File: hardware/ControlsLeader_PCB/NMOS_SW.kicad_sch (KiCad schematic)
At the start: 7 parts, among them Q15 NMOS

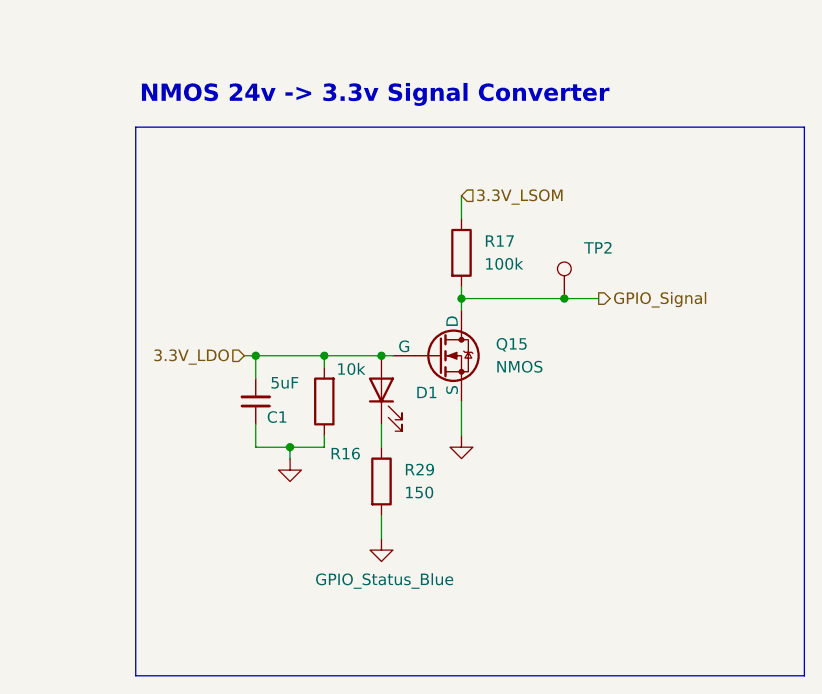
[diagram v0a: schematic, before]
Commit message: Schematic RevA
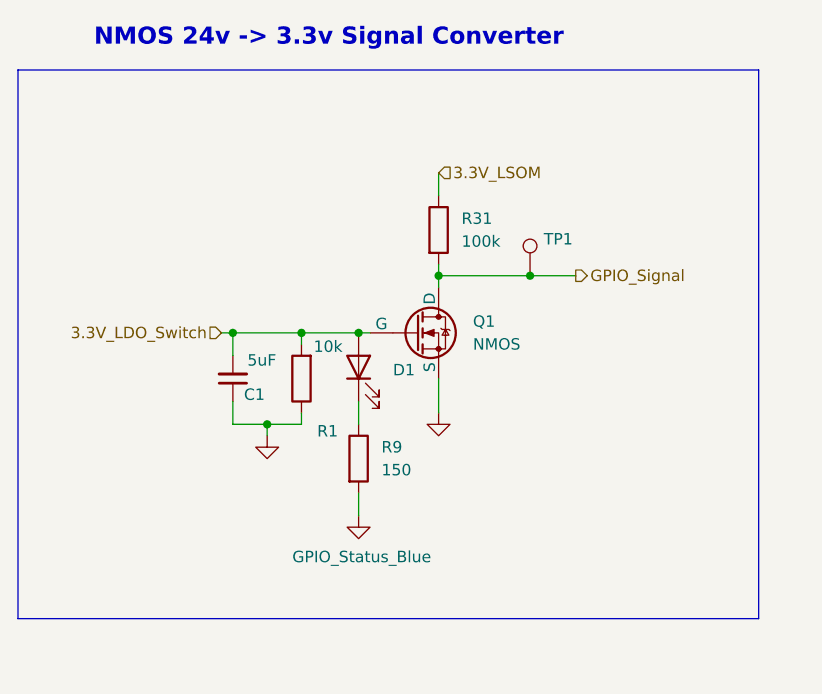
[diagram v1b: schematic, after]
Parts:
- removed Q15: NMOS, LSOM_IRLM:SOT23, symbol Simulation_SPICE:NMOS
- removed R16: 10k, Capacitor_SMD:C_0603_1608Metric_Pad1.08x0.95mm_HandSolder, symbol Device:R
- removed R17: 100k, Capacitor_SMD:C_0603_1608Metric_Pad1.08x0.95mm_HandSolder, symbol Device:R
- removed R29: 150, Capacitor_SMD:C_0603_1608Metric_Pad1.08x0.95mm_HandSolder, symbol Device:R
- removed TP2: TestPoint, TestPoint:TestPoint_Pad_1.0x1.0mm, symbol Connector:TestPoint
- added Q1: NMOS, LSOM_IRLM:SOT23, symbol Simulation_SPICE:NMOS
- added R1: 10k, Capacitor_SMD:C_0603_1608Metric_Pad1.08x0.95mm_HandSolder, symbol Device:R
- added R31: 100k, Capacitor_SMD:C_0603_1608Metric_Pad1.08x0.95mm_HandSolder, symbol Device:R
- added R9: 150, Capacitor_SMD:C_0603_1608Metric_Pad1.08x0.95mm_HandSolder, symbol Device:R
- added TP1: TestPoint, TestPoint:TestPoint_Pad_1.0x1.0mm, symbol Connector:TestPoint
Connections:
- net 3.3V_LSOM: now also R31.1
- net GND: now also Q1.3 (S), R1.1, R9.2
- net GPIO_Signal: now also Q1.1 (D), R31.2, TP1.1
- net at D1.1 (K): now also R9.1
- net 3.3V_LDO renamed 3.3V_LDO_Switch
- net 3.3V_LDO_Switch: now also Q1.2 (G), R1.2
